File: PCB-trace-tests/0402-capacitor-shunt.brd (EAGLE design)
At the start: 101.6 x 10.2 mm, 2 parts

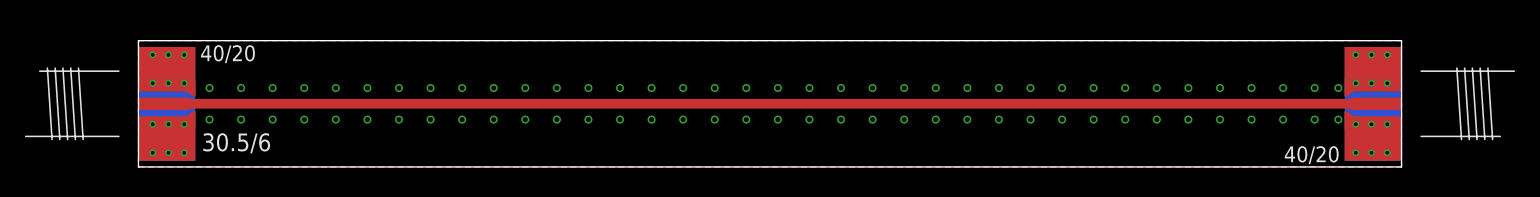
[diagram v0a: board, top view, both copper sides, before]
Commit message: checkpoint
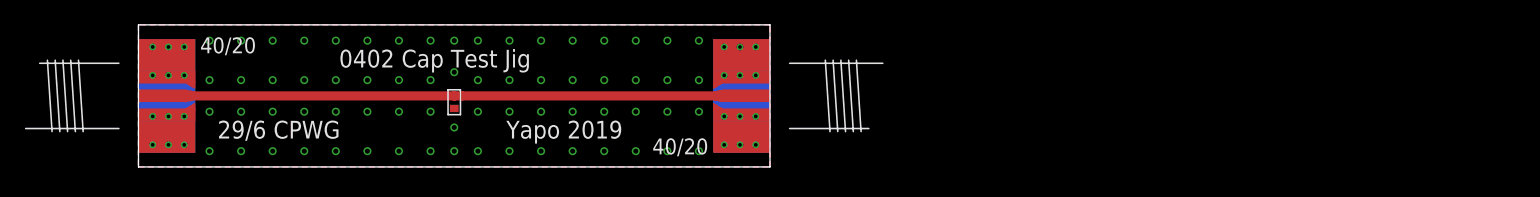
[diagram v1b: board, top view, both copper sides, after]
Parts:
- removed U$1, U$2: (no value), sma_footprint_2l:SMA_EDGE_LAUNCH_2L_4020_TAPER
- added C1: (no value), yapo:C0402
- added J1, J2: (no value), sma_footprint_2l:SMA_EDGE_LAUNCH_2L_4020_TAPER
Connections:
- net GND: now also C1.1, J1.BOTTOM_GND, J1.GND@1, J1.GND@14, J1.GND@15, J1.GND@16, J1.GND@17, J1.GND@2, J1.GND@3, J1.GND@4, J1.GND@5, J1.GND@6, J1.GND@7, J1.GND@8, J1.GND_PAD1, J1.GND_PAD2, J1.P$1, J1.P$2, J2.BOTTOM_GND, J2.GND@1, J2.GND@14, J2.GND@15, J2.GND@16, J2.GND@17, J2.GND@2, J2.GND@3, J2.GND@4, J2.GND@5, J2.GND@6, J2.GND@7, J2.GND@8, J2.GND_PAD1, J2.GND_PAD2, J2.P$1, J2.P$2; no longer U$1.BOTTOM_GND, U$1.GND@1, U$1.GND@14, U$1.GND@15, U$1.GND@16, U$1.GND@17, U$1.GND@2, U$1.GND@3, U$1.GND@4, U$1.GND@5, U$1.GND@6, U$1.GND@7, U$1.GND@8, U$1.GND_PAD1, U$1.GND_PAD2, U$1.P$1, U$1.P$2, U$2.BOTTOM_GND, U$2.GND@1, U$2.GND@14, U$2.GND@15, U$2.GND@16, U$2.GND@17, U$2.GND@2, U$2.GND@3, U$2.GND@4, U$2.GND@5, U$2.GND@6, U$2.GND@7, U$2.GND@8, U$2.GND_PAD1, U$2.GND_PAD2, U$2.P$1, U$2.P$2
- net N$1: now also C1.2, J1.CENTER@1, J2.CENTER@1; no longer U$1.CENTER@1, U$2.CENTER@1
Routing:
- net N$1: track 97.8 -> 45.9 mm
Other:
- board size 101.6 x 10.2 mm -> 50.8 x 11.4 mm
- board text added: "0402 Cap Test Jig"
- board text added: "29/6 CPWG"
- board text added: "Yapo 2019"
- board text removed: "30.5/6"
